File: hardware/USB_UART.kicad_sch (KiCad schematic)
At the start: 16 parts, among them Q17 BC847BS-7-F, Q28 NPN, Q29 NPN, SW1 SW_SPDT, U13 USB5926C, U14 CP2102N-QFN20

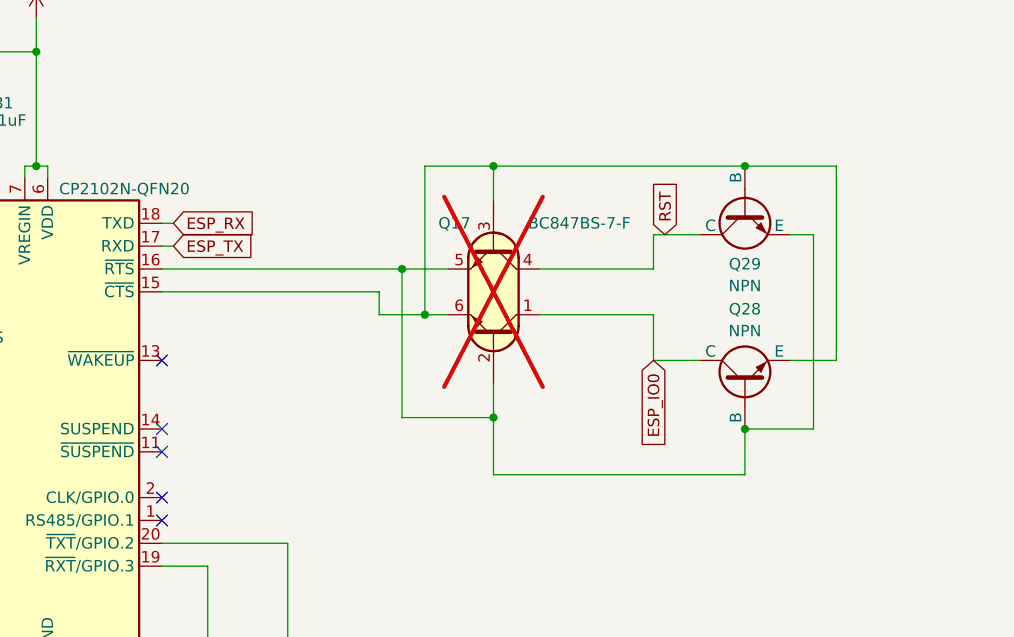
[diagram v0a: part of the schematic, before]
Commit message: working on usb pd protocol implimentation
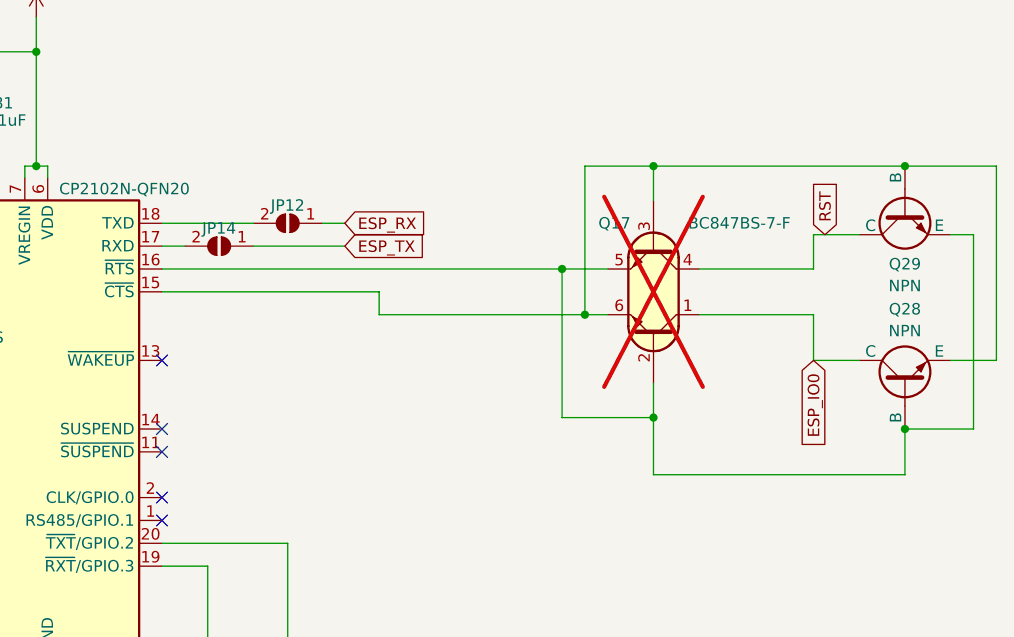
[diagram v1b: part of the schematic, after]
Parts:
- added JP12, JP14: ~, Jumper:SolderJumper-2_P1.3mm_Open_RoundedPad1.0x1.5mm, symbol Jumper:SolderJumper_2_Open
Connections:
- net ESP_RX: now also JP12.1 (A); no longer U14.18 (TXD)
- net ESP_TX: now also JP14.1 (A); no longer U14.17 (RXD)
- new net: JP14.2 (B), U14.17 (RXD)
- new net: JP12.2 (B), U14.18 (TXD)
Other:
- moved on the sheet: Q17, Q28, Q29
